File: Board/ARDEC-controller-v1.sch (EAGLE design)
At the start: 27 parts, among them IC1 L293D, IC2 L293D, IC4 MEGA8-P, IC5 7805T, Q2 16MHz

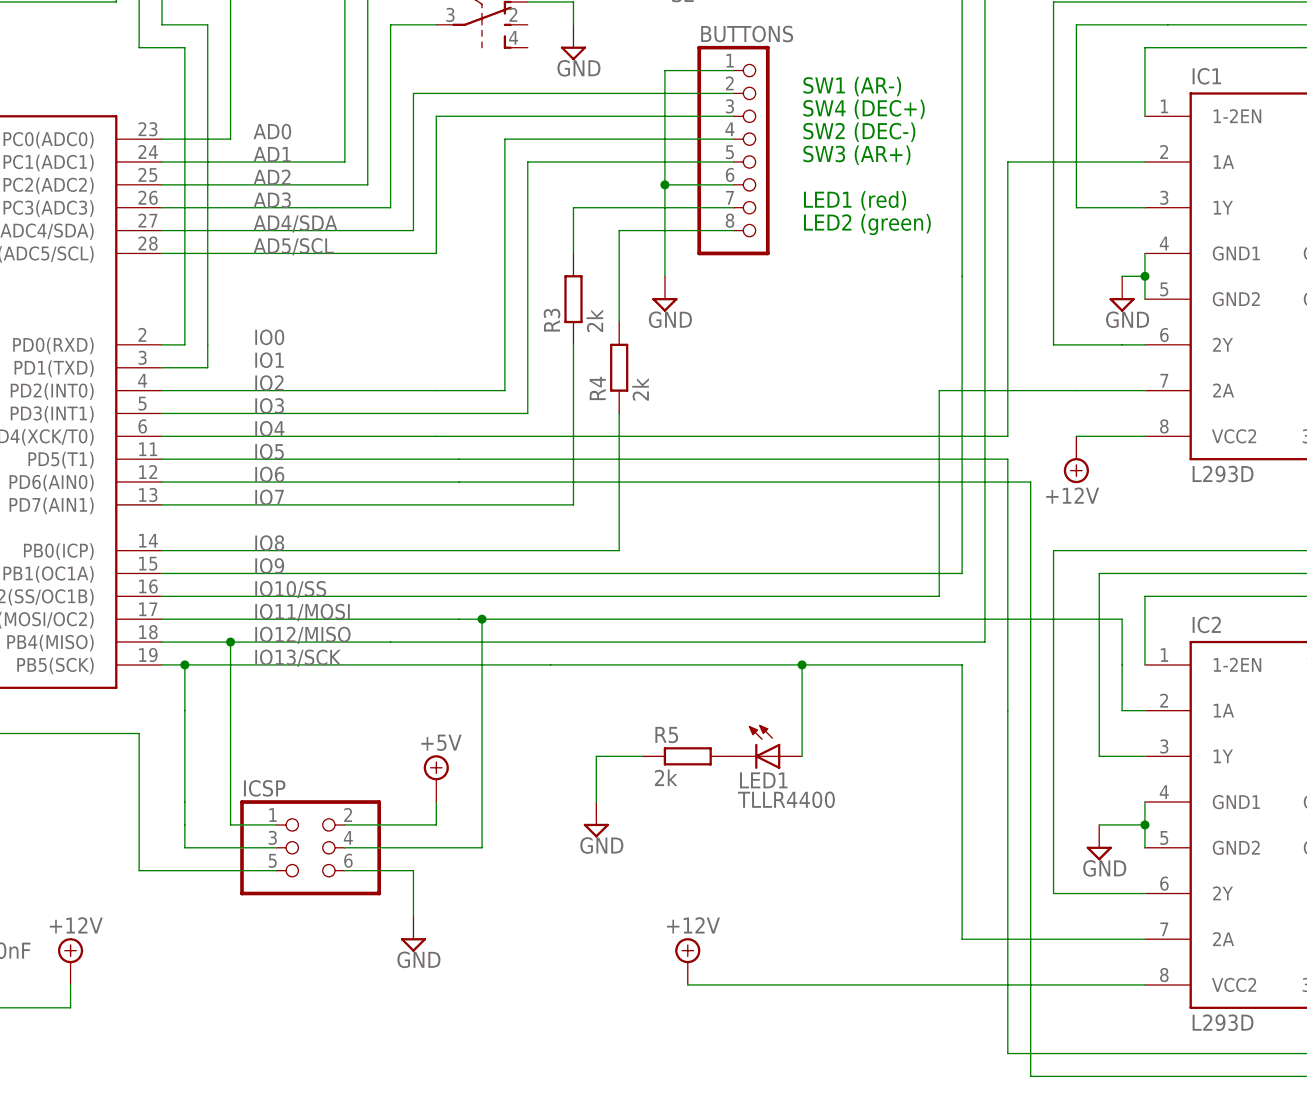
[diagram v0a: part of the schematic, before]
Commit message: Version 2.0
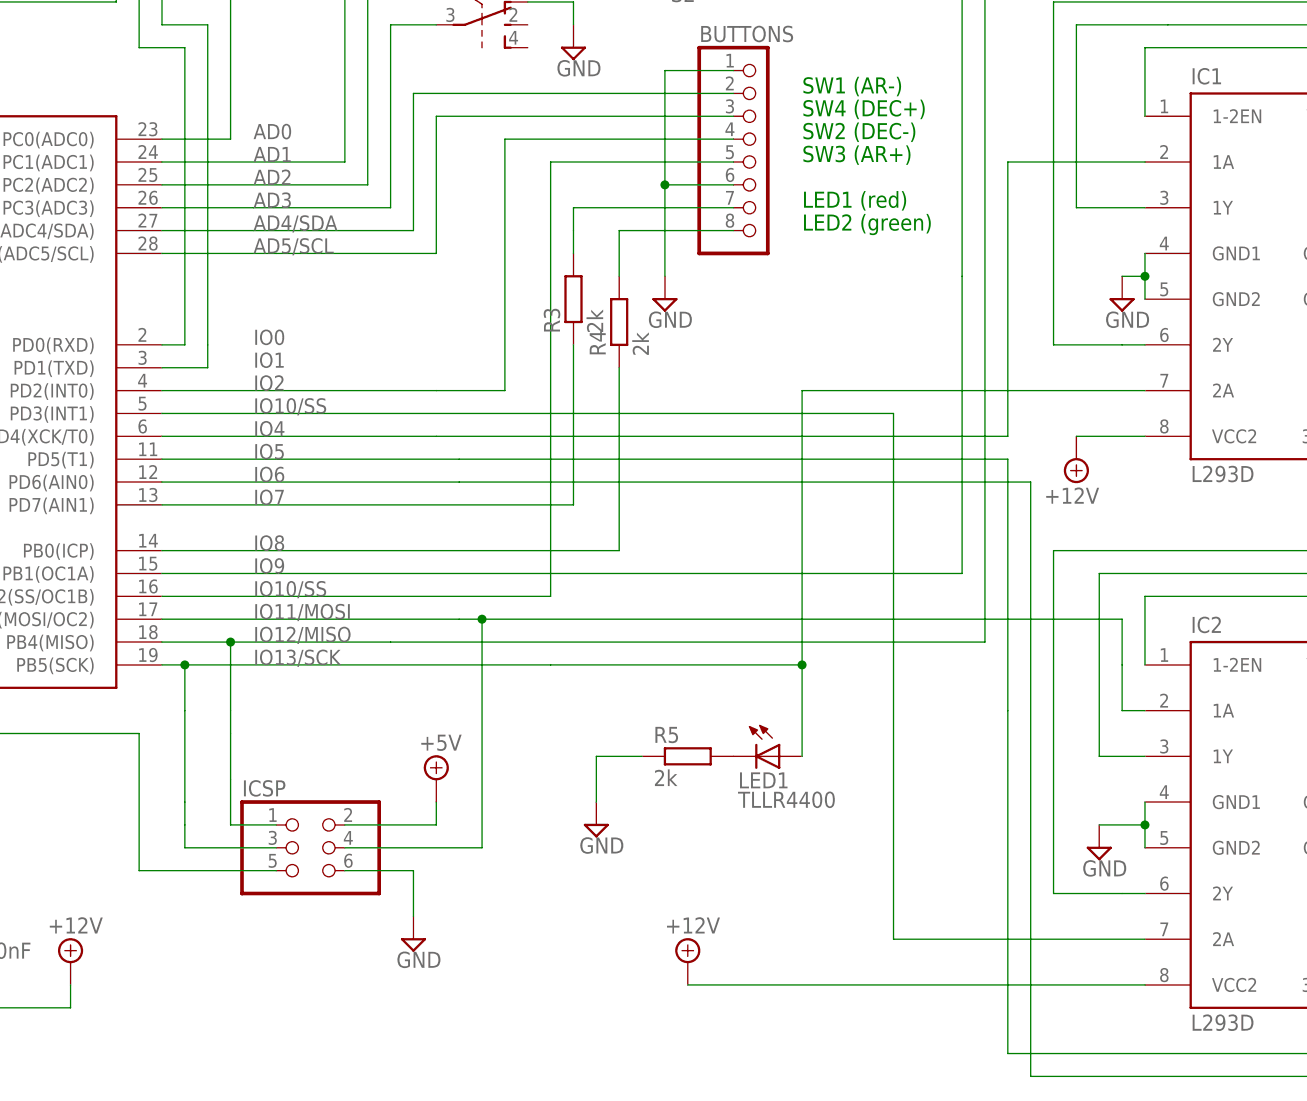
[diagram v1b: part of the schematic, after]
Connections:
- removed net IO3: BUTTONS.5, IC4.PD3(INT1)
- new net N$15: IC2.2A, IC4.PD3(INT1)
- net IO10/SS: now also BUTTONS.5; no longer IC1.2A
- net IO13/SCK: now also IC1.2A; no longer IC2.2A
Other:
- moved on the sheet: R4
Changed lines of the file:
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@@
 <?xml version="1.0" encoding="utf-8"?>
 <!DOCTYPE eagle SYSTEM "eagle.dtd">
-<eagle version="6.6.0">
+<eagle version="9.1.2">
 <drawing>
 <settings>
 <setting alwaysvectorfont="no"/>
+<setting keepoldvectorfont="yes"/>
 <setting verticaltext="up"/>
 </settings>
@@
 <instance part="SUPPLY11" gate="GND" x="71.12" y="60.96"/>
 <instance part="R3" gate="G$1" x="60.96" y="60.96" rot="R90"/>
-<instance part="R4" gate="G$1" x="66.04" y="53.34" rot="R90"/>
+<instance part="R4" gate="G$1" x="66.04" y="58.42" rot="R90"/>
 <instance part="D2" gate="1" x="-38.1" y="-10.16" rot="R90"/>
 <instance part="C4" gate="G$1" x="-7.62" y="-7.62"/>
@@
 </segment>
 </net>
-<net name="IO3" class="0">
-<segment>
-<pinref part="IC4" gate="G$1" pin="PD3(INT1)"/>
-<wire x1="15.24" y1="48.26" x2="55.88" y2="48.26" width="0.1524" layer="91"/>
-<wire x1="55.88" y1="48.26" x2="55.88" y2="76.2" width="0.1524" layer="91"/>
-<label x="25.4" y="48.26" size="1.6764" layer="95"/>
-<pinref part="BUTTONS" gate="A" pin="5"/>
-<wire x1="55.88" y1="76.2" x2="78.74" y2="76.2" width="0.1524" layer="91"/>
-</segment>
-</net>
 <net name="IO2" class="0">
 <segment>
@@
 <label x="25.4" y="33.02" size="1.6764" layer="95"/>
 <pinref part="R4" gate="G$1" pin="1"/>
-<wire x1="66.04" y1="33.02" x2="66.04" y2="48.26" width="0.1524" layer="91"/>
+<wire x1="66.04" y1="33.02" x2="66.04" y2="53.34" width="0.1524" layer="91"/>
 </segment>
 </net>
@@
 <segment>
 <pinref part="R4" gate="G$1" pin="2"/>
-<wire x1="66.04" y1="58.42" x2="66.04" y2="68.58" width="0.1524" layer="91"/>
+<wire x1="66.04" y1="63.5" x2="66.04" y2="68.58" width="0.1524" layer="91"/>
 <pinref part="BUTTONS" gate="A" pin="8"/>
 <wire x1="66.04" y1="68.58" x2="78.74" y2="68.58" width="0.1524" layer="91"/>
@@
 </segment>
 </net>
-<net name="IO10/SS" class="0">
-<segment>
-<pinref part="IC1" gate="G$1" pin="2A"/>
-<wire x1="116.84" y1="50.8" x2="124.46" y2="50.8" width="0.1524" layer="91"/>
-<wire x1="101.6" y1="50.8" x2="116.84" y2="50.8" width="0.1524" layer="91"/>
-<pinref part="IC4" gate="G$1" pin="PB2(SS/OC1B)"/>
-<wire x1="15.24" y1="27.94" x2="101.6" y2="27.94" width="0.1524" layer="91"/>
-<label x="25.4" y="27.94" size="1.6764" layer="95"/>
-<wire x1="101.6" y1="50.8" x2="101.6" y2="27.94" width="0.1524" layer="91"/>
-</segment>
-</net>
 <net name="IO7" class="0">
 <segment>
@@
 <segment>
 <pinref part="ICSP" gate="A" pin="3"/>
-<wire x1="104.14" y1="20.32" x2="86.36" y2="20.32" width="0.1524" layer="91"/>
 <pinref part="IC4" gate="G$1" pin="PB5(SCK)"/>
 <wire x1="86.36" y1="20.32" x2="58.42" y2="20.32" width="0.1524" layer="91"/>
@@
 <pinref part="LED1" gate="G$1" pin="A"/>
 <wire x1="86.36" y1="20.32" x2="86.36" y2="10.16" width="0.1524" layer="91"/>
+<pinref part="IC1" gate="G$1" pin="2A"/>
+<wire x1="124.46" y1="50.8" x2="86.36" y2="50.8" width="0.1524" layer="91"/>
+<wire x1="86.36" y1="50.8" x2="86.36" y2="20.32" width="0.1524" layer="91"/>
 <junction x="86.36" y="20.32"/>
-<wire x1="104.14" y1="20.32" x2="104.14" y2="-10.16" width="0.1524" layer="91"/>
-<pinref part="IC2" gate="G$1" pin="2A"/>
-<wire x1="104.14" y1="-10.16" x2="124.46" y2="-10.16" width="0.1524" layer="91"/>
 </segment>
 </net>
@@
 </segment>
 </net>
+<net name="N$15" class="0">
+<segment>
+<pinref part="IC4" gate="G$1" pin="PD3(INT1)"/>
+<wire x1="15.24" y1="48.26" x2="96.52" y2="48.26" width="0.1524" layer="91"/>
+<wire x1="96.52" y1="48.26" x2="96.52" y2="-10.16" width="0.1524" layer="91"/>
+<pinref part="IC2" gate="G$1" pin="2A"/>
+<wire x1="96.52" y1="-10.16" x2="124.46" y2="-10.16" width="0.1524" layer="91"/>
+</segment>
+</net>
+<net name="IO10/SS" class="0">
+<segment>
+<label x="25.4" y="48.26" size="1.6764" layer="95"/>
+<pinref part="IC4" gate="G$1" pin="PB2(SS/OC1B)"/>
+<wire x1="15.24" y1="27.94" x2="58.42" y2="27.94" width="0.1524" layer="91"/>
+<label x="25.4" y="27.94" size="1.6764" layer="95"/>
+<wire x1="58.42" y1="76.2" x2="58.42" y2="27.94" width="0.1524" layer="91"/>
+<pinref part="BUTTONS" gate="A" pin="5"/>
+<wire x1="58.42" y1="76.2" x2="78.74" y2="76.2" width="0.1524" layer="91"/>
+</segment>
+</net>
